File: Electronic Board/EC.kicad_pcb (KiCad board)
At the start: 4 copper layers, 170.2 x 130 mm, 101 parts, among them J1 NMJ4HCD2, J2 4840.2201, J3 173950578, J4 NMJ4HCD2, J5 NMJ4HCD2, J6 NMJ4HCD2, J8 Conn_02x07_Odd_Even, SW2 SW_SPDT, U2 BU18SD2MG-MTR, U4 SGTL5000XNAA3, U5 IS42S16400J-xC, U502 BU33SD5WG-TR, U6 STM32F446ZCTx

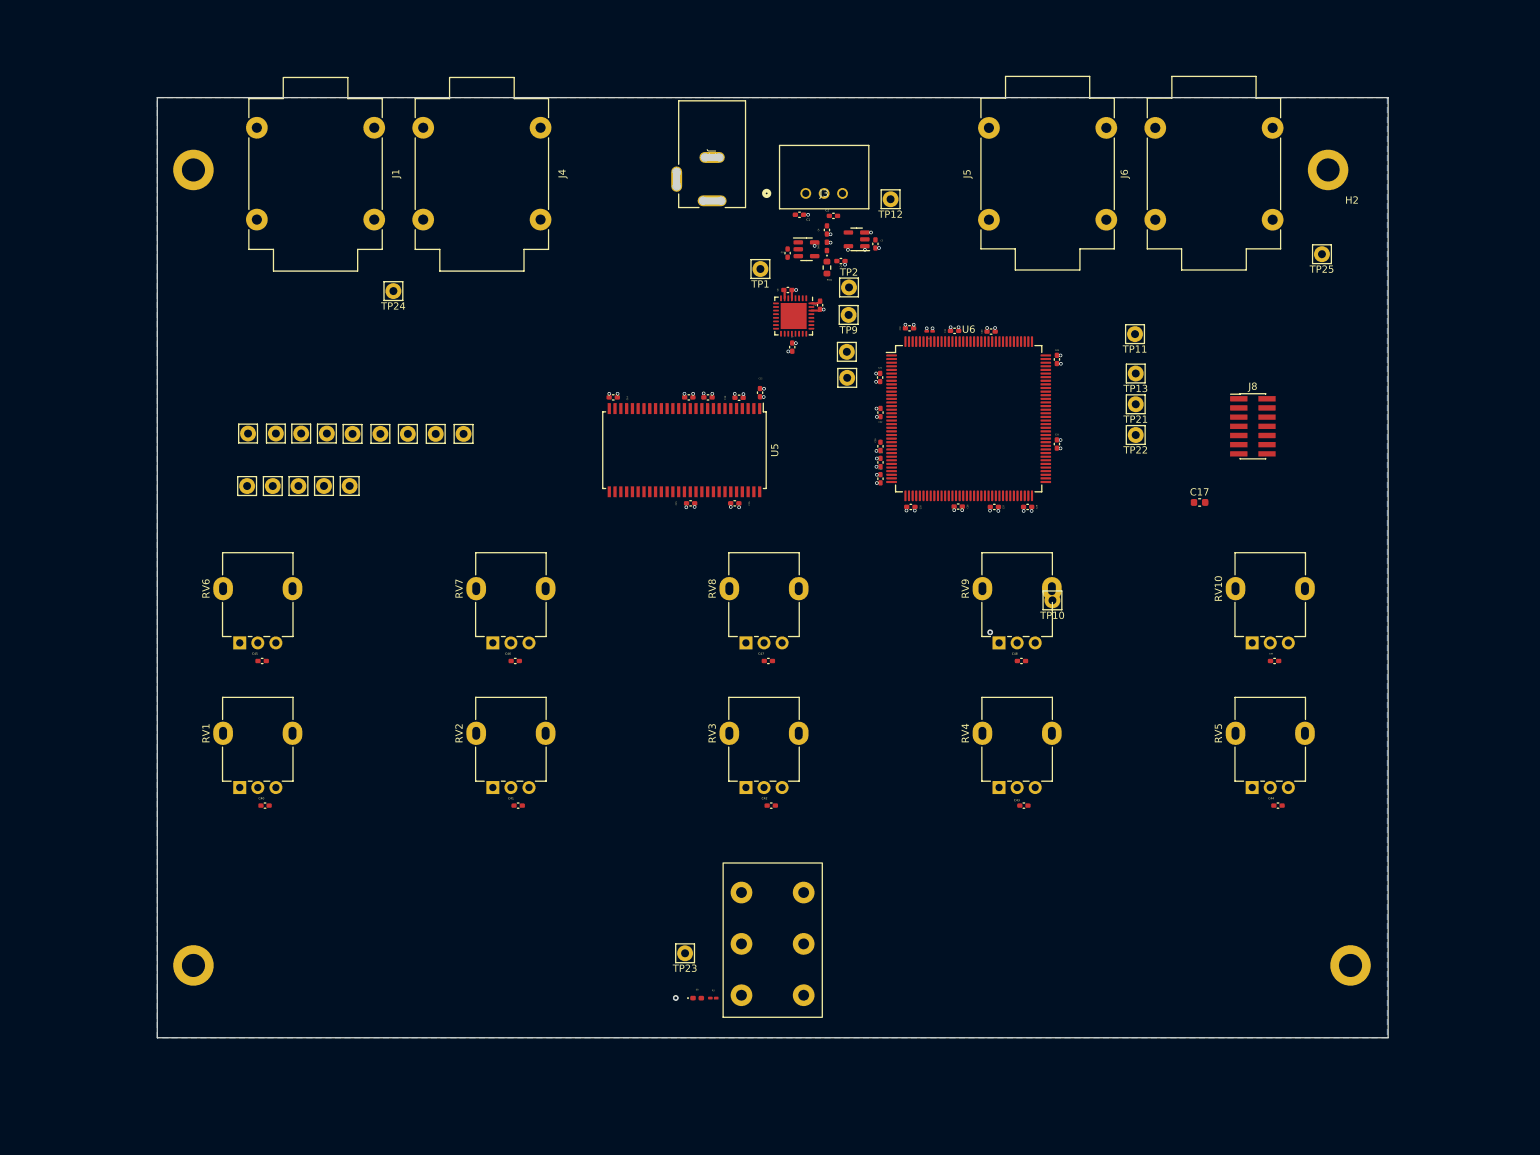
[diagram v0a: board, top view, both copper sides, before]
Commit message: Add files via upload
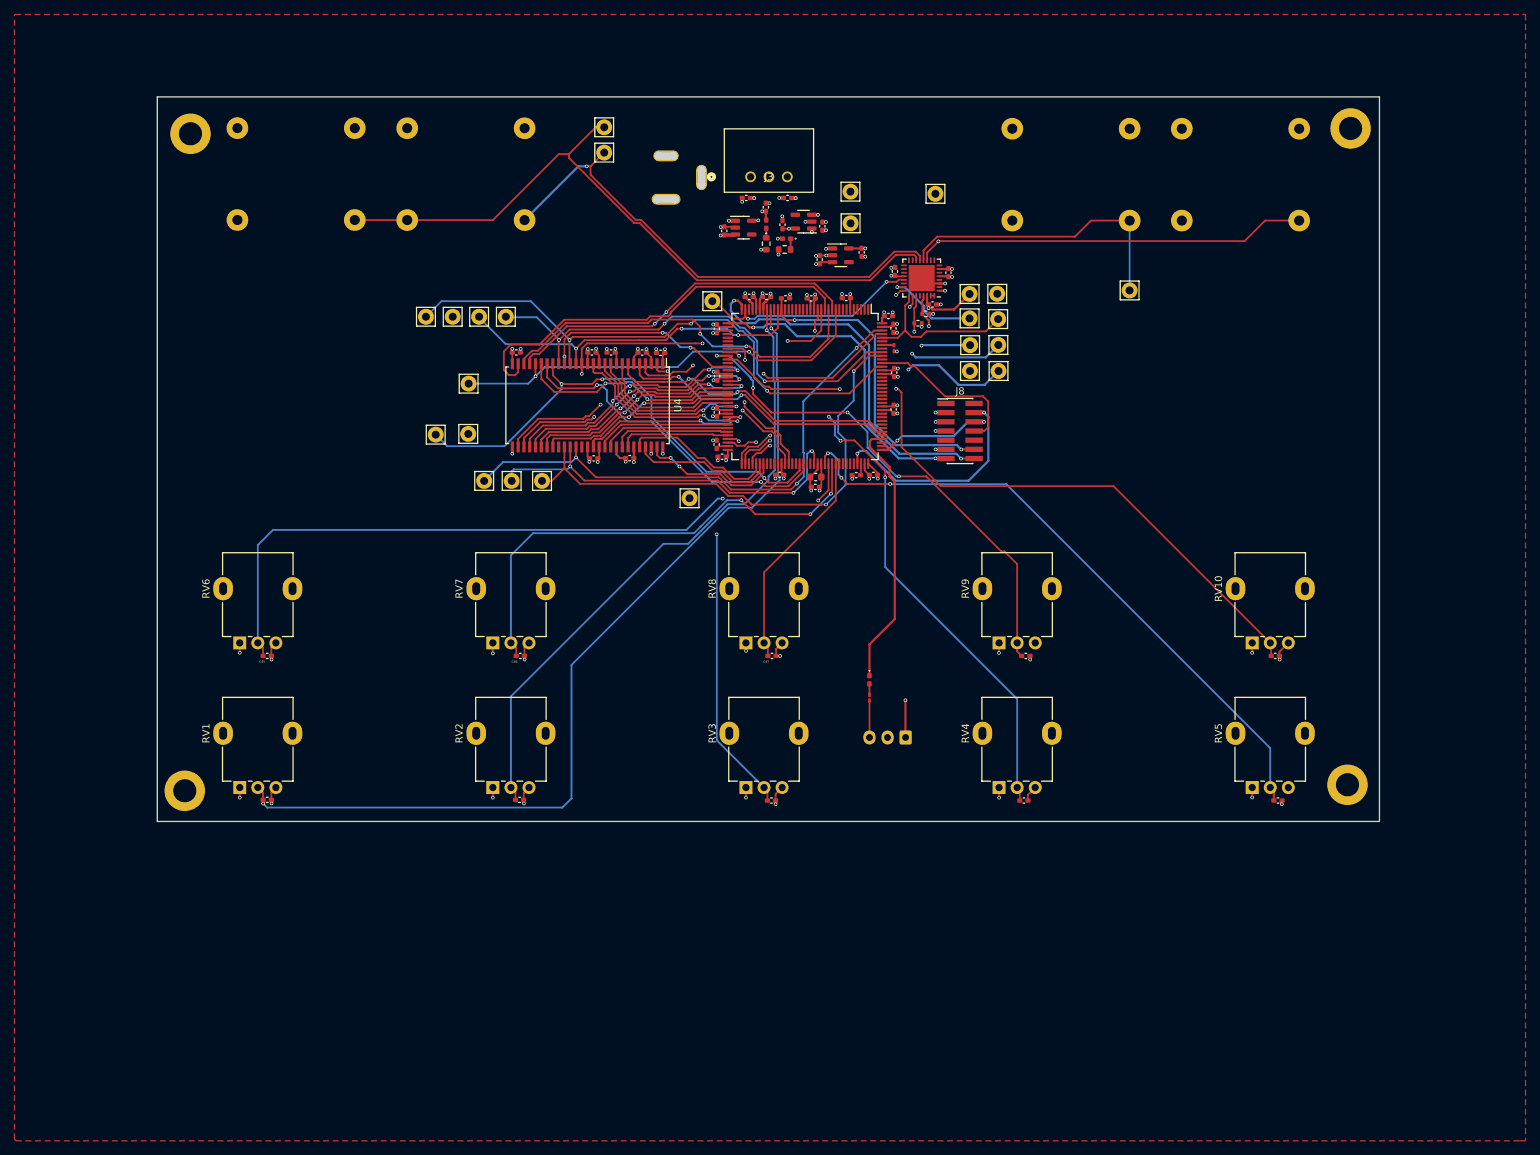
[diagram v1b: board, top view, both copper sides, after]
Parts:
- removed C16: 100nF, Capacitor_SMD:C_0402_1005Metric_Pad0.74x0.62mm_HandSolder
- removed D502: RED, LED_SMD:LED_0402_1005Metric_Pad0.77x0.64mm_HandSolder
- removed R502: 1k, Resistor_SMD:R_0603_1608Metric
- removed RAM_A0, RAM_DQ, SDNE, TP7: TestPoint, Connector_Pin:Pin_D1.1mm_L8.5mm_W2.5mm_FlatFork
- removed SW2: SW_SPDT, Library:RS_Pro_SPDT_8466720
- removed U5: IS42S16400J-xC, Package_SO:TSOP-II-54_22.2x10.16mm_P0.8mm
- removed U502: BU33SD5WG-TR, Package_TO_SOT_SMD:SOT-23-5
- added C18: 2.2uF, Capacitor_SMD:C_0402_1005Metric_Pad0.74x0.62mm_HandSolder, F.Cu at (102.3, 68.0)
- added C19: 2.2uF, Capacitor_SMD:C_0402_1005Metric_Pad0.74x0.62mm_HandSolder, F.Cu at (121.7, 72.2)
- added C34: 100nF, Capacitor_SMD:C_0402_1005Metric_Pad0.74x0.62mm_HandSolder, F.Cu at (109.2, 47.5)
- added C35: 100nF, Capacitor_SMD:C_0402_1005Metric_Pad0.74x0.62mm_HandSolder, F.Cu at (126.8, 51.9)
- added C50: 100nF, Capacitor_SMD:C_0402_1005Metric_Pad0.74x0.62mm_HandSolder, F.Cu at (134.4, 44.2)
- added C51: 100nF, Capacitor_SMD:C_0402_1005Metric_Pad0.74x0.62mm_HandSolder, F.Cu at (132.2, 48.6)
- added C60: 100nF, Capacitor_SMD:C_0402_1005Metric_Pad0.74x0.62mm_HandSolder, F.Cu at (111.9, 47.8)
- added D1: RED, LED_SMD:LED_0402_1005Metric_Pad0.77x0.64mm_HandSolder, F.Cu at (109.2, 37.5)
- added D3: RED, LED_SMD:LED_0402_1005Metric_Pad0.77x0.64mm_HandSolder, F.Cu at (112.0, 39.5)
- added J9: Conn_01x03, Connector_JST:JST_XH_S3B-XH-A-1_1x03_P2.50mm_Horizontal, B.Cu at (128.5, 108.5)
- added R2: 1k, Resistor_SMD:R_0603_1608Metric, F.Cu at (111.8, 41.0)
- added R5: 1.5k, Resistor_SMD:R_0402_1005Metric, F.Cu at (130.2, 51.2)
- added R6: 510, Resistor_SMD:R_0201_0603Metric_Pad0.64x0.40mm_HandSolder, F.Cu at (126.9, 54.6)
- added R7: 1.5k, Resistor_SMD:R_0402_1005Metric, F.Cu at (131.3, 49.9)
- added TP34: TestPoint, Connector_Pin:Pin_D1.1mm_L8.5mm_W2.5mm_FlatFork, F.Cu at (86.8, 27.6)
- added TP35: TestPoint, Connector_Pin:Pin_D1.1mm_L8.5mm_W2.5mm_FlatFork, F.Cu at (132.6, 33.3)
- added U1: BU33SD5WG-TR, Package_TO_SOT_SMD:SOT-23-5, F.Cu at (106.1, 38.0)
- added U3: BU18SD2MG-MTR, Package_TO_SOT_SMD:SOT-23-5, F.Cu at (119.5, 41.8)
- added U7: SGTL5000XNAA3, Package_DFN_QFN:QFN-32-1EP_5x5mm_P0.5mm_EP3.6x3.6mm, F.Cu at (130.7, 45.0)
- C7, C8: value 100nF -> 1uF
- J1, J2, J4, J5, J6: moved to B.Cu
- R1: value 510 -> 1k; footprint Resistor_SMD:R_0201_0603Metric_Pad0.64x0.40mm_HandSolder -> Resistor_SMD:R_0603_1608Metric
- U2: value BU18SD2MG-MTR -> BU33SD5WG-TR
- U4: value SGTL5000XNAA3 -> IS42S16400J-xC; footprint Package_DFN_QFN:QFN-32-1EP_5x5mm_P0.5mm_EP3.6x3.6mm -> Package_SO:TSOP-II-54_22.2x10.16mm_P0.8mm
- moved TP25 125.1 mm to (63.5, 66.6)
- moved TP13 98.5 mm to (62.1, 50.3), turned to 180 degrees
- moved TP23 96.2 mm to (137.3, 50.5)
- moved TP11 94.4 mm to (65.8, 50.3), turned to 180 degrees
- moved TP4 90.9 mm to (137.3, 47.1), turned to 180 degrees
- moved TP10 85.2 mm to (73.2, 50.3)
- moved TP24 84.4 mm to (141.3, 57.8)
- moved TP3 81.3 mm to (120.9, 37.4), turned to 180 degrees
- moved TP20 78.2 mm to (137.4, 57.8), turned to 0 degrees
- moved TP18 69.2 mm to (101.8, 48.1), turned to 0 degrees
- moved TP5 62.1 mm to (86.8, 24.1), turned to 180 degrees
- moved TP12 59.2 mm to (69.5, 50.3)
- moved TP17 57.7 mm to (98.6, 75.4), turned to 0 degrees
- moved C17 53.2 mm to (116.0, 72.5), turned to 180 degrees
- moved D2 50.1 mm to (123.5, 100.5), turned to -90 degrees
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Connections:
- net Buffer renamed Net-(D2-K)
- C20 pad 1: NRST -> +3.3V
- C24 pad 1: +3.3V -> +3.3VA
- C5 pad 1: +3.3V -> +5V
- C6 pad 1: +1V8 -> +3.3VA
- C8 pad 1: +3.3V -> +1V8
- C9 pad 1: +1V8 -> +3.3V
- J1 pad T: Ve_guitare_L -> /Codec/Ve_guitare_L
- J4 pad T: Ve_guitare_R -> /Codec/Ve_guitare_R
- J4 pad TN: Ve_guitare_L -> /Codec/Ve_guitare_L
- J5 pad T: Vs_guitare_L -> /Codec/Vs_guitare_L
- J5 pad TN: GND -> unconnected-(J5-PadTN)
- J6 pad T: Vs_guitare_R -> /Codec/Vs_guitare_R
- J6 pad TN: Vs_guitare_L -> unconnected-(J6-PadTN)
- R1 pad 1: GND -> Net-(D1-K)
- R1 pad 2: Vs_3,3V -> GND
- TP1 pad 1: +3.3V -> +5V
- TP10 pad 1: Ve_guitare_R -> /STM32/SDNE1 
- TP11 pad 1: Vs_guitare_R -> /STM32/SDNRAS
- TP12 pad 1: +5V -> /STM32/SDNWE
- TP13 pad 1: SDNE1 -> /STM32/SDNCAS
- TP14 pad 1: SDCKE1 -> /STM32/NBL0
- TP15 pad 1: SDCLK -> /STM32/A0
- TP16 pad 1: NBL0 -> /STM32/NBL1
- TP17 pad 1: NBL1 -> /STM32/D0
- TP18 pad 1: SDNWE -> /Codec/SYS_MCLK
- TP19 pad 1: SDNCAS -> /Codec/SDA_I2C
- TP2 pad 1: +1V8 -> +3.3V
- TP20 pad 1: SDNRAS -> /Codec/SCL_I2C
- TP21 pad 1: A0 -> /Codec/SD_I2S
- TP22 pad 1: D0 -> /Codec/DOUT_I2S
- TP23 pad 1: Net-(D2-A) -> /Codec/WS_I2S
- TP24 pad 1: Ve_guitare_L -> /Codec/CK_I2S
- TP25 pad 1: Vs_guitare_L -> /STM32/BA0
- TP3 pad 1: SYS_MCLK -> +3.3VA
- TP4 pad 1: WS_I2S -> +1V8
- TP5 pad 1: CK_I2S -> /Codec/Ve_guitare_L
- TP6 pad 1: DOUT_I2S -> /Codec/Vs_guitare_L
- TP8 pad 1: SDA_I2C -> /STM32/SDCLK
- TP9 pad 1: SCL_I2C -> /STM32/SDCKE1
- U2 pad 1: +3.3V -> +5V
- U2 pad 3: +3.3V -> +5V
- U2 pad 5: +1V8 -> +3.3VA
- U4 pad 1: GND -> +3.3V
- U4 pad 10: unconnected-(U4-VAG-Pad10) -> /STM32/D5
- U4 pad 11: Vs_guitare_R -> /STM32/D6
- U4 pad 12: Vs_guitare_L -> GND
- U4 pad 13: Ve_guitare_R -> /STM32/D7
- U4 pad 14: Ve_guitare_L -> +3.3V
- U4 pad 15: unconnected-(U4-MIC-Pad15) -> /STM32/NBL0
- U4 pad 16: unconnected-(U4-MIC_BIAS-Pad16) -> /STM32/SDNWE
- U4 pad 17: unconnected-(U4-NC-Pad17) -> /STM32/SDNCAS
- U4 pad 18: unconnected-(U4-CPFILT-Pad18) -> /STM32/SDNRAS
- U4 pad 19: unconnected-(U4-NC-Pad19) -> /STM32/SDNE1 
- U4 pad 2: unconnected-(U4-HP_R-Pad2) -> /STM32/D0
- U4 pad 20: +3.3V -> /STM32/BA0
- U4 pad 21: SYS_MCLK -> /STM32/BA1
- U4 pad 22: unconnected-(U4-NC-Pad22) -> /STM32/A10
- U4 pad 23: WS_I2S -> /STM32/A0
- U4 pad 24: CK_I2S -> /STM32/A1
- U4 pad 25: DOUT_I2S -> /STM32/A2
- U4 pad 26: SD_I2S -> /STM32/A3
- U4 pad 27: SDA_I2C -> +3.3V
- U4 pad 28: unconnected-(U4-NC-Pad28) -> GND
- U4 pad 29: SCL_I2C -> /STM32/A4
- U4 pad 3: GND -> +3.3V
- U4 pad 30: +1V8 -> /STM32/A5
- U4 pad 31: GND -> /STM32/A6
- U4 pad 32: GND -> /STM32/A7
- U4 pad 33: GND -> /STM32/A8
- U4 pad 4: unconnected-(U4-HP_VGND-Pad4) -> /STM32/D1
- U4 pad 5: +3.3V -> /STM32/D2
- U4 pad 6: unconnected-(U4-HP_L-Pad6) -> GND
- U4 pad 7: GND -> /STM32/D3
- U4 pad 8: unconnected-(U4-NC-Pad8) -> /STM32/D4
- U4 pad 9: unconnected-(U4-NC-Pad9) -> +3.3V
- U6 pad 10: A0 -> /STM32/A0
- U6 pad 106: unconnected-(U6-VCAP_2-Pad106) -> Net-(U6-VCAP_2)
- U6 pad 11: A1 -> /STM32/A1
- U6 pad 111: Pot_8 -> unconnected-(U6-PC10-Pad111)
- U6 pad 114: D2 -> /STM32/D2
- U6 pad 115: D3 -> /STM32/D3
- U6 pad 12: A2 -> /STM32/A2
- U6 pad 13: A3 -> /STM32/A3
- U6 pad 132: SDNCAS -> /STM32/SDNCAS
- U6 pad 135: SDCKE1 -> /STM32/SDCKE1
- U6 pad 136: SDNE1 -> /STM32/SDNE1 
- U6 pad 138: Vs_3,3V -> Net-(U6-BOOT0)
- U6 pad 14: A4 -> /STM32/A4
- U6 pad 140: DOUT_I2S -> /Codec/DOUT_I2S
- U6 pad 141: NBL0 -> /STM32/NBL0
- U6 pad 142: NBL1 -> /STM32/NBL1
- U6 pad 143: unconnected-(U6-PDR_ON-Pad143) -> +3.3V
- U6 pad 15: A5 -> /STM32/A5
- U6 pad 23: /stm32/OSC_IN -> unconnected-(U6-PH0-Pad23)
- U6 pad 24: /stm32/OSC_OUT -> unconnected-(U6-PH1-Pad24)
- U6 pad 26: SDNWE -> /STM32/SDNWE
- U6 pad 32: unconnected-(U6-VREF+-Pad32) -> GND
- U6 pad 33: +3.3V -> +3.3VA
- U6 pad 35: SYS_MCLK -> /Codec/SYS_MCLK
- U6 pad 48: /stm32/BOOT1 -> unconnected-(U6-PB2-Pad48)
- U6 pad 49: SDNRAS -> /STM32/SDNRAS
- U6 pad 50: A6 -> /STM32/A6
- U6 pad 53: A7 -> /STM32/A7
- U6 pad 54: A8 -> /STM32/A8
- U6 pad 55: A9 -> /STM32/A9
- U6 pad 56: A10 -> /STM32/A10
- U6 pad 57: A11 -> /STM32/A11
- U6 pad 58: D4 -> /STM32/D4
- U6 pad 59: D5 -> /STM32/D5
- U6 pad 60: D6 -> /STM32/D6
- U6 pad 63: D7 -> /STM32/D7
- U6 pad 64: D8 -> /STM32/D8
- U6 pad 65: D9 -> /STM32/D9
- U6 pad 66: D10 -> /STM32/D10
- U6 pad 67: D11 -> /STM32/D11
- U6 pad 68: D12 -> /STM32/D12
- U6 pad 69: SCL_I2C -> /Codec/SCL_I2C
- U6 pad 70: SDA_I2C -> /Codec/SDA_I2C
- U6 pad 71: unconnected-(U6-VCAP_1-Pad71) -> Net-(U6-VCAP_1)
- U6 pad 73: WS_I2S -> /Codec/WS_I2S
- U6 pad 74: CK_I2S -> /Codec/CK_I2S
- U6 pad 76: SD_I2S -> /Codec/SD_I2S
- U6 pad 77: D13 -> /STM32/D13
- U6 pad 78: D14 -> /STM32/D14
- U6 pad 79: D15 -> /STM32/D15
- U6 pad 8: /stm32/OSC32_IN -> unconnected-(U6-PC14-Pad8)
- U6 pad 85: D0 -> /STM32/D0
- U6 pad 86: D1 -> /STM32/D1
- U6 pad 89: BA0 -> /STM32/BA0
- U6 pad 9: /stm32/OSC32_OUT -> unconnected-(U6-PC15-Pad9)
- U6 pad 90: BA1 -> /STM32/BA1
- U6 pad 93: SDCLK -> /STM32/SDCLK
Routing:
- net Pot_0: track 0.00 -> 127.3 mm, vias 0 -> 2
- net Pot_5: track 0.00 -> 102.0 mm, vias 0 -> 2
- net /Codec/Ve_guitare_L: track 0.00 -> 98.6 mm
- net Pot_9: track 0.00 -> 97.5 mm, vias 1 -> 2
- net Pot_4: track 0.00 -> 88.3 mm, vias 0 -> 3
- net Pot_1: track 0.00 -> 87.0 mm, vias 0 -> 1
- net Pot_3: track 0.00 -> 85.2 mm, vias 0 -> 4
- net /Codec/SCL_I2C: track 0.00 -> 81.1 mm, vias 0 -> 2
- net /STM32/SDNCAS: track 0.00 -> 79.3 mm, vias 0 -> 3
- net /STM32/NBL1: track 0.00 -> 75.0 mm, vias 0 -> 3
- net +3.3V: track 1.16 -> 75.4 mm, vias 28 -> 40
- net GND: track 2.53 -> 76.8 mm, vias 23 -> 58
- net /STM32/SDCKE1: track 0.00 -> 70.7 mm, vias 0 -> 2
- net Pot_8: track 0.00 -> 70.4 mm, vias 0 -> 4
- net /STM32/NBL0: track 0.00 -> 70.4 mm, vias 0 -> 3
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- added copper zone on In2.Cu, net +3.3VA
- added copper zone on F.Cu, net GND
- removed copper zone on In1.Cu, net +5V
- removed copper zone on B.Cu, net GND
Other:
- board size 170.2 x 130 mm -> 169 x 100.2 mm
